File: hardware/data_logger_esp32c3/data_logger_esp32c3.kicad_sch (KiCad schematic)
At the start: 74 parts, among them U1 ESP32-C3-MINI-1, U10 A03401A, U11 SX1509BIULTRT, U2 AZ1117IH-3.3TRG1, U4 LM321MF, U5 LM321MF, U6 LM321MF, U7 LM321MF, U8 LM321MF, U9 A03401A

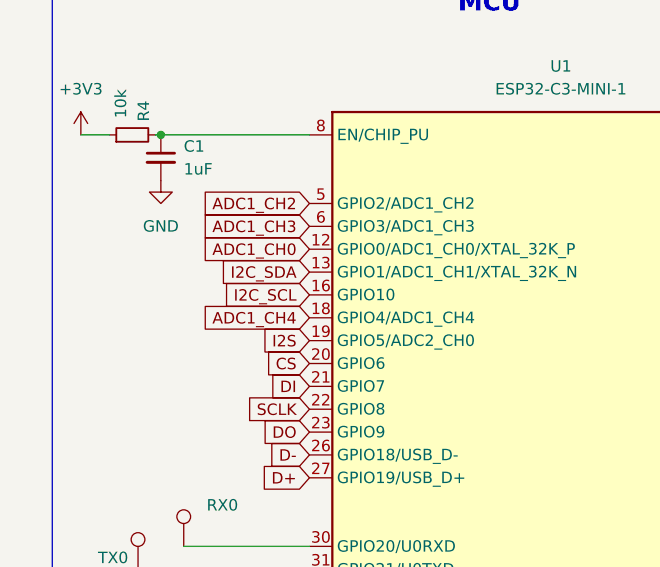
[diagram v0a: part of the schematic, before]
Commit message: more layout
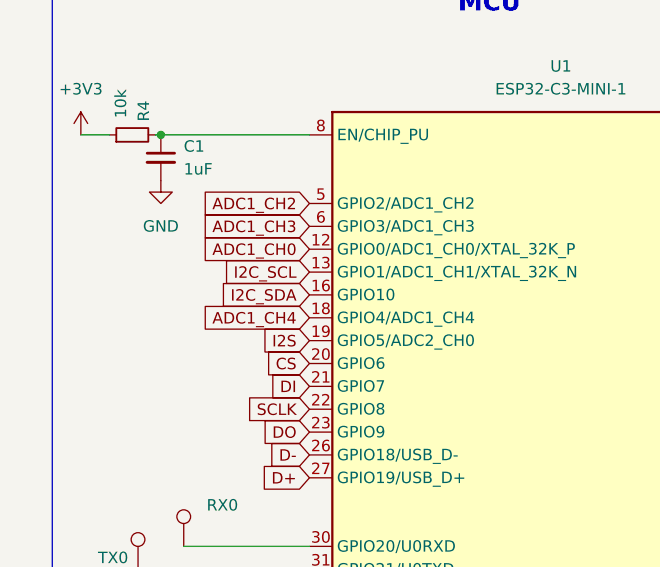
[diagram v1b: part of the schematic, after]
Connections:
- net I2C_SCL: now also U1.13 (GPIO1/ADC1_CH1/XTAL_32K_N); no longer U1.16 (GPIO10)
- net I2C_SDA: now also U1.16 (GPIO10); no longer U1.13 (GPIO1/ADC1_CH1/XTAL_32K_N)
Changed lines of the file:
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@@
+    )
+  )
+  (global_label "I2C_SDA" (shape input) (at 55.245 61.595 180) (fields_autoplaced)
+    (effects (font (size 1.27 1.27)) (justify right))
+    (property "Intersheet References" "${INTERSHEET_REFS}" (id 0) (at 45.2119 61.5156 0)
+      (effects (font (size 1.27 1.27)) (justify right) hide)
     )
   )
@@
     )
   )
-  (global_label "I2C_SCL" (shape input) (at 55.245 61.595 180) (fields_autoplaced)
-    (effects (font (size 1.27 1.27)) (justify right))
-    (property "Intersheet References" "${INTERSHEET_REFS}" (id 0) (at 45.2724 61.5156 0)
-      (effects (font (size 1.27 1.27)) (justify right) hide)
-    )
-  )
   (global_label "SCLK" (shape input) (at 46.99 185.42 180) (fields_autoplaced)
     (effects (font (size 1.27 1.27)) (justify right))
@@
     (effects (font (size 1.27 1.27)) (justify right))
     (property "Intersheet References" "${INTERSHEET_REFS}" (id 0) (at 130.3019 152.9556 0)
+      (effects (font (size 1.27 1.27)) (justify right) hide)
+    )
+  )
+  (global_label "I2C_SCL" (shape input) (at 55.245 59.055 180) (fields_autoplaced)
+    (effects (font (size 1.27 1.27)) (justify right))
+    (property "Intersheet References" "${INTERSHEET_REFS}" (id 0) (at 45.2724 58.9756 0)
       (effects (font (size 1.27 1.27)) (justify right) hide)
     )
@@
       (effects (font (size 1.27 1.27)) (justify right) hide)
     )
-  )
-  (global_label "I2C_SDA" (shape input) (at 55.245 59.055 180) (fields_autoplaced)
-    (effects (font (size 1.27 1.27)) (justify right))
-    (property "Intersheet References" "${INTERSHEET_REFS}" (id 0) (at 45.2119 58.9756 0)
-      (effects (font (size 1.27 1.27)) (justify right) hide)
-    )
